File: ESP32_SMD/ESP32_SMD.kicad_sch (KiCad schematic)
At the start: 31 parts, among them J1 POWER, J10 INPUT_2, J11 Conn_01x15_Socket, J12 Conn_01x02_Socket, J13 Conn_01x02_Socket, J14 Conn_01x02_Socket, J15 Conn_01x02_Socket, J17 I2C, J18 Conn_01x03_Socket, J19 Conn_01x03_Socket, J2 Conn_01x02_Socket, J3 Serial Converter, J4 I2C, J5 Conn_01x02_Socket, J6 Conn_01x02_Socket, J7 Conn_01x02_Socket, J8 Conn_01x02_Socket, J9 INPUT_1, SW1 SW_Nidec_CAS-120A1, SW2 SW_DPST_x2, SW3 SW_DPST_x2, U1 ESP32-WROOM-32E, U2 R-78B1.2-2.0

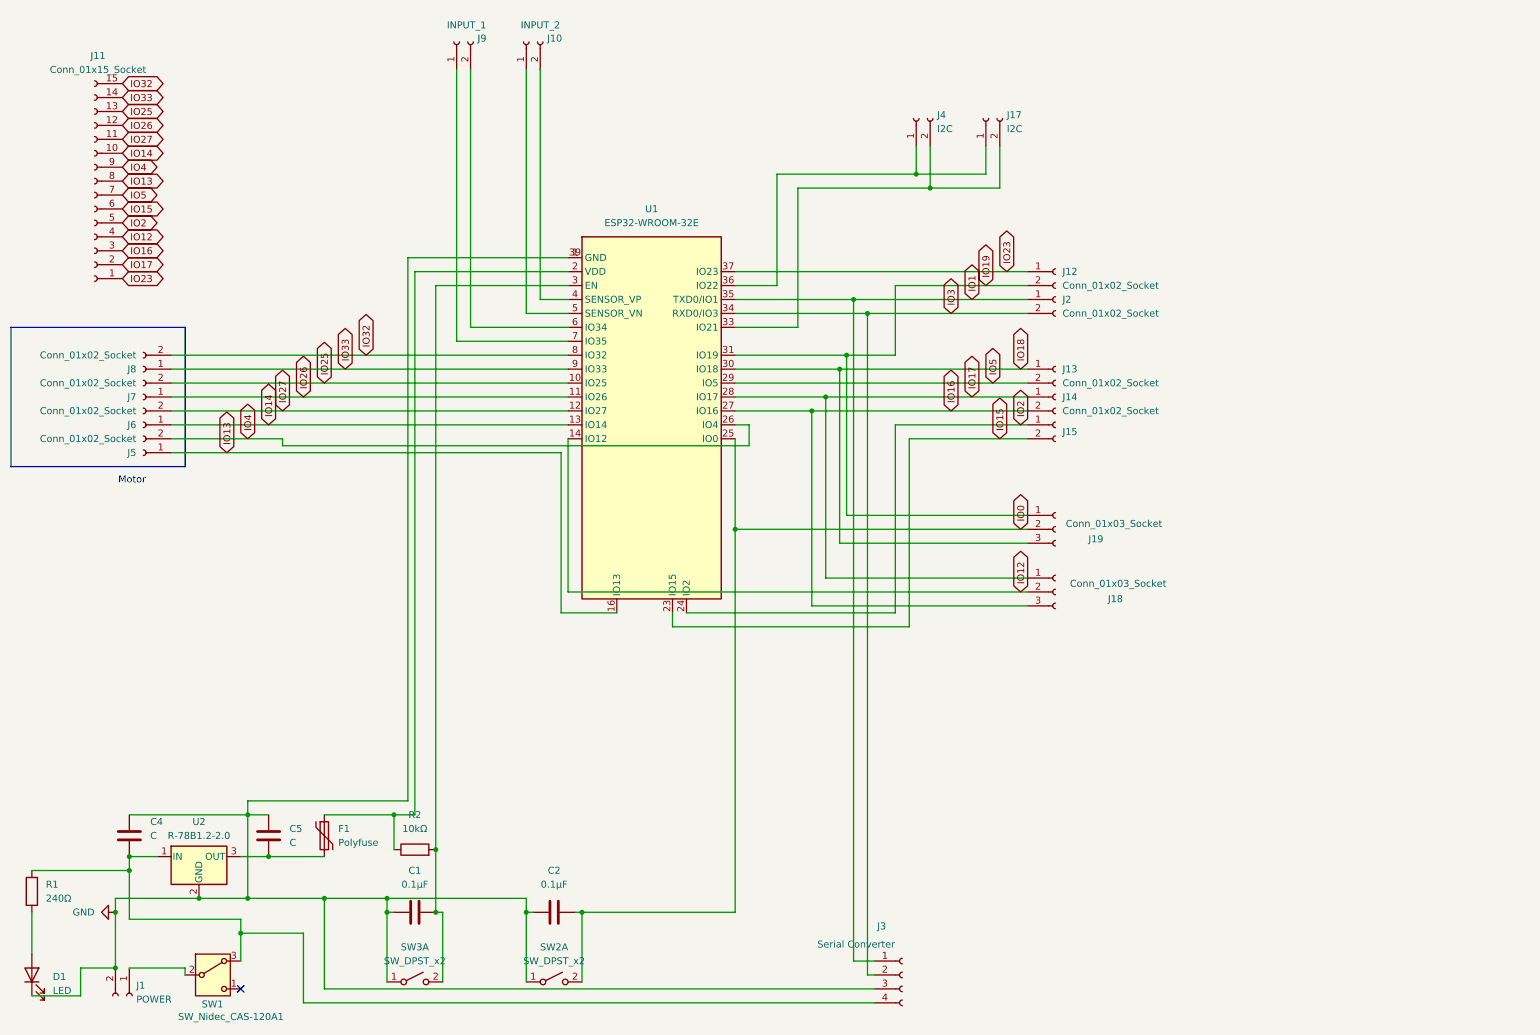
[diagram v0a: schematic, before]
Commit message: 2024/11/05
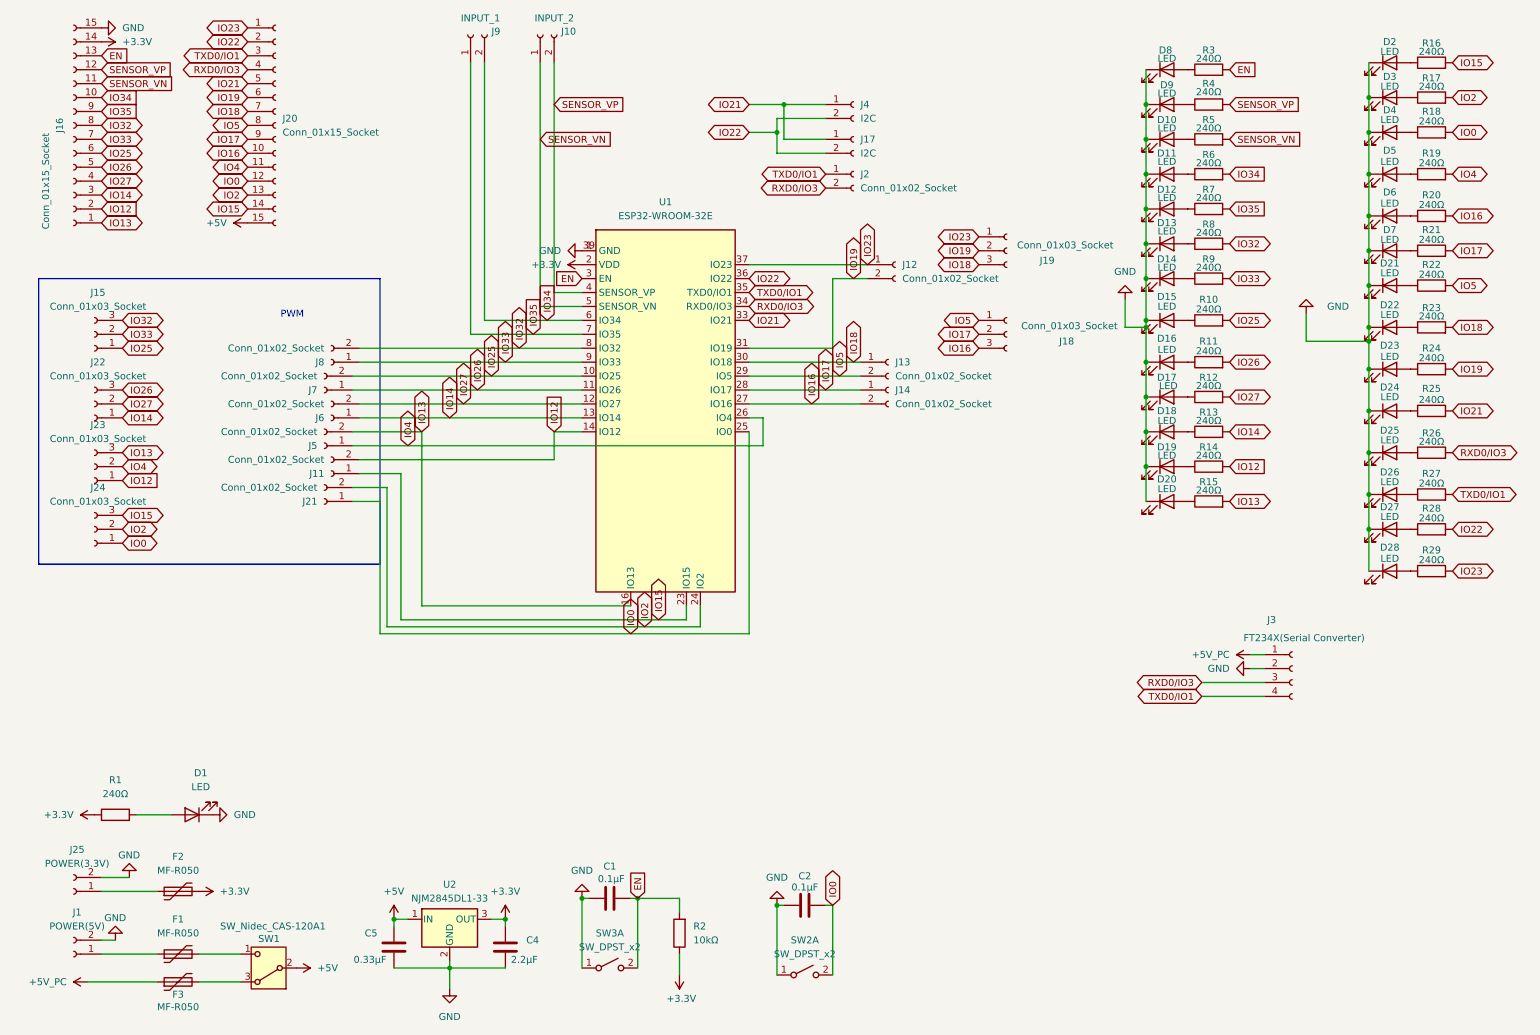
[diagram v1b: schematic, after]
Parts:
- removed J11: Conn_01x15_Socket, Connector_Dsub:DSUB-15_Female_Vertical_P2.77x2.84mm, symbol Connector:Conn_01x15_Socket
- removed J15: Conn_01x02_Socket, Connector_JST:JST_XH_B2B-XH-A_1x02_P2.50mm_Vertical, symbol Connector:Conn_01x02_Socket
- added D10, D11, D12, D13, D14, D15, D16, D17, D18, D19, D2, D20, D21, D22, D23, D24, D25, D26, D27, D28, D3, D4, D5, D6, D7, D8, D9: LED, LED_SMD:LED_0603_1608Metric_Pad1.05x0.95mm_HandSolder, symbol Device:LED
- added F2, F3: MF-R050, 00a:MF-R050, symbol Device:Polyfuse
- added J11, J21: Conn_01x02_Socket, Connector_JST:JST_XH_B2B-XH-A_1x02_P2.50mm_Vertical, symbol Connector:Conn_01x02_Socket
- added J15, J22, J23, J24: Conn_01x03_Socket, Connector_JST:JST_XH_B3B-XH-A_1x03_P2.50mm_Vertical, symbol Connector:Conn_01x03_Socket
- added J16, J20: Conn_01x15_Socket, Connector_PinHeader_2.54mm:PinHeader_1x15_P2.54mm_Vertical, symbol Connector:Conn_01x15_Socket
- added J25: POWER(3.3V), Connector_JST:JST_XH_B2B-XH-A_1x02_P2.50mm_Vertical, symbol Connector:Conn_01x02_Socket
- added R10, R11, R12, R13, R14, R15, R16, R17, R18, R19, R20, R21, R22, R23, R24, R25, R26, R27, R28, R29, R3, R4, R5, R6, R7, R8, R9: 240Ω, Resistor_SMD:R_0603_1608Metric_Pad0.98x0.95mm_HandSolder, symbol Device:R
- C1, C2: footprint Capacitor_THT:C_Disc_D3.0mm_W2.0mm_P2.50mm -> Capacitor_SMD:C_0603_1608Metric_Pad1.08x0.95mm_HandSolder
- C4: value C -> 2.2μF; footprint Connector_PinHeader_2.54mm:PinHeader_1x02_P2.54mm_Vertical -> Capacitor_SMD:C_0603_1608Metric_Pad1.08x0.95mm_HandSolder
- C5: value C -> 0.33μF; footprint Connector_PinHeader_2.54mm:PinHeader_1x02_P2.54mm_Vertical -> Capacitor_SMD:C_0603_1608Metric_Pad1.08x0.95mm_HandSolder
- D1: footprint LED_THT:LED_D3.0mm_Horizontal_O6.35mm_Z10.0mm -> LED_SMD:LED_0603_1608Metric
- F1: value Polyfuse -> MF-R050; footprint 00a:RXEF005 -> 00a:MF-R050
- J1: value POWER -> POWER(5V)
- J3: value Serial Converter -> FT234X(Serial Converter)
- R1, R2: footprint Resistor_THT:R_Axial_DIN0207_L6.3mm_D2.5mm_P10.16mm_Horizontal -> Resistor_SMD:R_0603_1608Metric_Pad0.98x0.95mm_HandSolder
- U2: value R-78B1.2-2.0 -> NJM2845DL1-33; footprint Converter_DCDC:Converter_DCDC_RECOM_R-78B-2.0_THT -> 00a:TO-252-3_TabPin2
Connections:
- net GND: now also C4.1, C5.1, J3.2 (GND), D10.1 (K), D11.1 (K), D12.1 (K), D13.1 (K), D14.1 (K), D15.1 (K), D16.1 (K), D17.1 (K), D18.1 (K), D19.1 (K), D2.1 (K), D20.1 (K), D21.1 (K), D22.1 (K), D23.1 (K), D24.1 (K), D25.1 (K), D26.1 (K), D27.1 (K), D28.1 (K), D3.1 (K), D4.1 (K), D5.1 (K), D6.1 (K), D7.1 (K), D8.1 (K), D9.1 (K), J16.15 (Pin_15), J25.2 (Pin_2); no longer C4.2, C5.2, J3.3 (Pin_3)
- net IO0: now also J20.12 (Pin_12), J21.1 (Pin_1), J24.1 (Pin_1), R18.2; no longer J19.2 (Pin_2)
- net IO12: now also J11.2 (Pin_2), J16.2 (Pin_2), J23.1 (Pin_1), R14.2; no longer J18.2 (Pin_2)
- net IO13: now also J5.2 (Pin_2), J16.1 (Pin_1), J23.3 (Pin_3), R15.2; no longer J5.1 (Pin_1)
- net IO14: now also J16.3 (Pin_3), J22.1 (Pin_1), R13.2
- net IO15: now also J11.1 (Pin_1), J20.14 (Pin_14), J24.3 (Pin_3), R16.2
- net IO16: now also J20.10 (Pin_10), R20.2
- net IO17: now also J18.2 (Pin_2), J20.9 (Pin_9), R21.2; no longer J18.1 (Pin_1)
- net IO18: now also J20.7 (Pin_7), R23.2
- net IO19: now also J19.2 (Pin_2), J20.6 (Pin_6), R24.2; no longer J19.1 (Pin_1)
- net IO2: now also J20.13 (Pin_13), J21.2 (Pin_2), J24.2 (Pin_2), R17.2
- net IO23: now also J19.1 (Pin_1), J20.1 (Pin_1), R29.2
- net IO25: now also J15.1 (Pin_1), J16.6 (Pin_6), R10.2
- net IO26: now also J16.5 (Pin_5), J22.3 (Pin_3), R11.2
- net IO27: now also J16.4 (Pin_4), J22.2 (Pin_2), R12.2
- net IO32: now also J15.3 (Pin_3), J16.8 (Pin_8), R8.2
- net IO33: now also J15.2 (Pin_2), J16.7 (Pin_7), R9.2
- net IO4: now also J5.1 (Pin_1), J20.11 (Pin_11), J23.2 (Pin_2), R19.2; no longer J5.2 (Pin_2)
- net IO5: now also J18.1 (Pin_1), J20.8 (Pin_8), R22.2
- net EN: now reaches C1.1, R2.2, SW3.2 (B), U1.3 (EN)
- net EN: now also J16.13 (Pin_13), R3.2
- net IO35: now reaches J9.1 (Pin_1), U1.7 (IO35)
- net IO35: now also J16.9 (Pin_9), R7.2
- net IO34: now reaches J9.2 (Pin_2), U1.6 (IO34)
- net IO34: now also J16.10 (Pin_10), R6.2
- net IO21: now reaches J17.1 (Pin_1), J4.1 (Pin_1)
- net IO21: now also U1.33 (IO21), J20.5 (Pin_5), R25.2; no longer U1.36 (IO22)
- net IO22: now reaches J17.2 (Pin_2), J4.2 (Pin_2)
- net IO22: now also U1.36 (IO22), J20.2 (Pin_2), R28.2; no longer U1.33 (IO21)
- net SENSOR_VN: now reaches J10.1 (Pin_1), U1.5 (SENSOR_VN)
- net SENSOR_VN: now also J16.11 (Pin_11), R5.2
- net SENSOR_VP: now reaches J10.2 (Pin_2), U1.4 (SENSOR_VP)
- net SENSOR_VP: now also J16.12 (Pin_12), R4.2
- net at D1.2 (A): now also R1.2; no longer R1.1
- net at J1.1 (Pin_1): now also F1.1; no longer SW1.2 (B)
- net +3.3V: now reaches R2.1, U1.2 (VDD)
- net +3.3V: now also C4.2, R1.1, U2.3 (OUT), F2.2, J16.14 (Pin_14); no longer F1.1
- net at SW1.1 (C): now also F1.2
- net IO1 renamed TXD0/IO1
- net TXD0/IO1: now also J3.4 (RxD), J20.3 (Pin_3), R27.2; no longer J3.1 (Pin_1)
- net IO3 renamed RXD0/IO3
- net RXD0/IO3: now also J3.3 (TxD), J20.4 (Pin_4), R26.2; no longer J3.2 (Pin_2)
- new net: D28.2 (A), R29.1
- new net: D7.2 (A), R21.1
- new net: D6.2 (A), R20.1
- new net: D23.2 (A), R24.1
- new net: D2.2 (A), R16.1
- new net: D8.2 (A), R3.1
- new net: D20.2 (A), R15.1
- new net: D13.2 (A), R8.1
- new net: D18.2 (A), R13.1
- new net: D25.2 (A), R26.1
- new net: D16.2 (A), R11.1
- new net: D27.2 (A), R28.1
- new net: D4.2 (A), R18.1
- new net: D15.2 (A), R10.1
- new net: F3.2, SW1.3 (A)
- new net: D21.2 (A), R22.1
- new net: F2.1, J25.1 (Pin_1)
- new net: D22.2 (A), R23.1
- new net: D24.2 (A), R25.1
- new net: D26.2 (A), R27.1
- new net: D17.2 (A), R12.1
- new net: D12.2 (A), R7.1
- new net: D10.2 (A), R5.1
- new net: D11.2 (A), R6.1
- new net: D9.2 (A), R4.1
- new net: D3.2 (A), R17.1
- new net: D14.2 (A), R9.1
- new net: D19.2 (A), R14.1
- new net: D5.2 (A), R19.1
- new net +5V: C5.2, J20.15 (Pin_15), SW1.2 (B), U2.1 (IN)
- new net +5V_PC: F3.1, J3.1 (5V)
- no-connect marks 1 -> 0
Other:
- note added: "PWM"
- note removed: "Motor"
- moved on the sheet: C1, C2, C4, C5, D1, F1, J1, J10, J12, J13, J14, J17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
